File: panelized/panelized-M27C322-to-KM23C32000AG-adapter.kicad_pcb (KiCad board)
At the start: 2 copper layers, 115.5 x 108 mm, 544 parts, among them J1 PinSocket_2x22_P1.27mm_Vertic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, U1 KM23C32000AG-adaptor

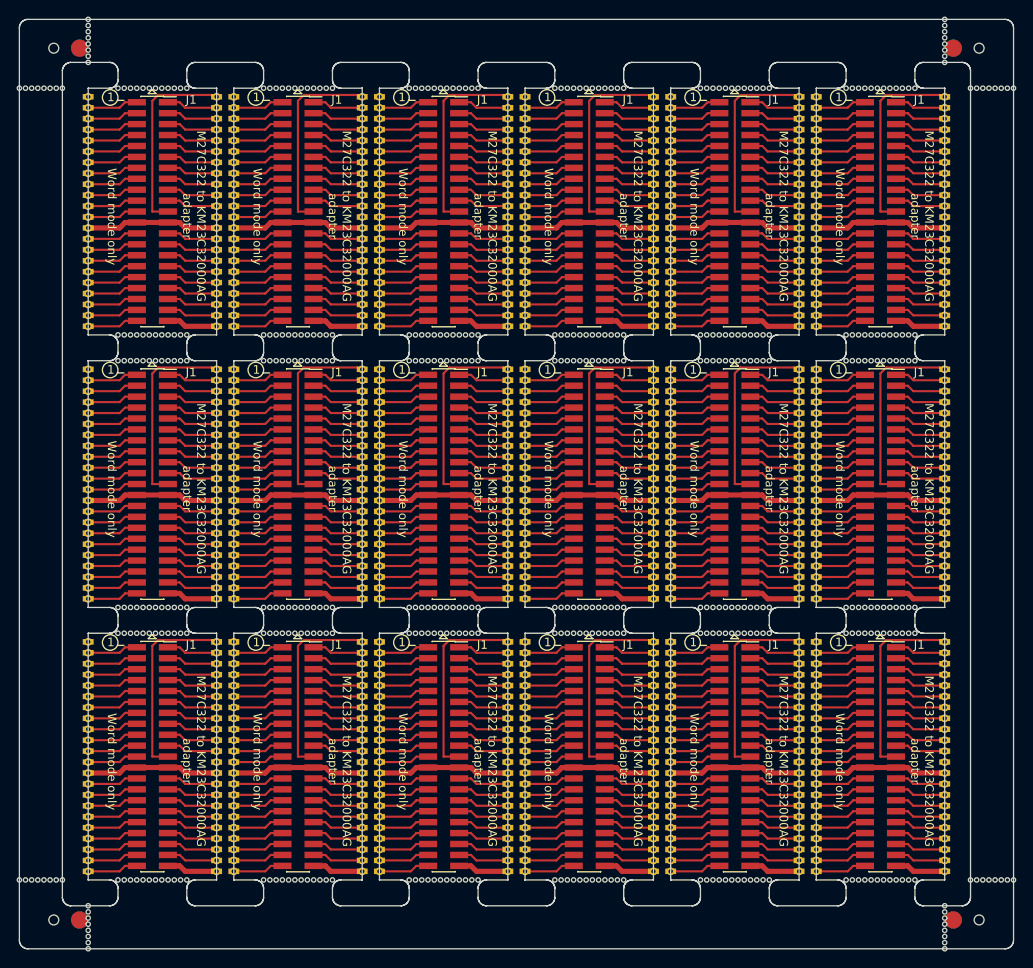
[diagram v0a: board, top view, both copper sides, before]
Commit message: WIP changes
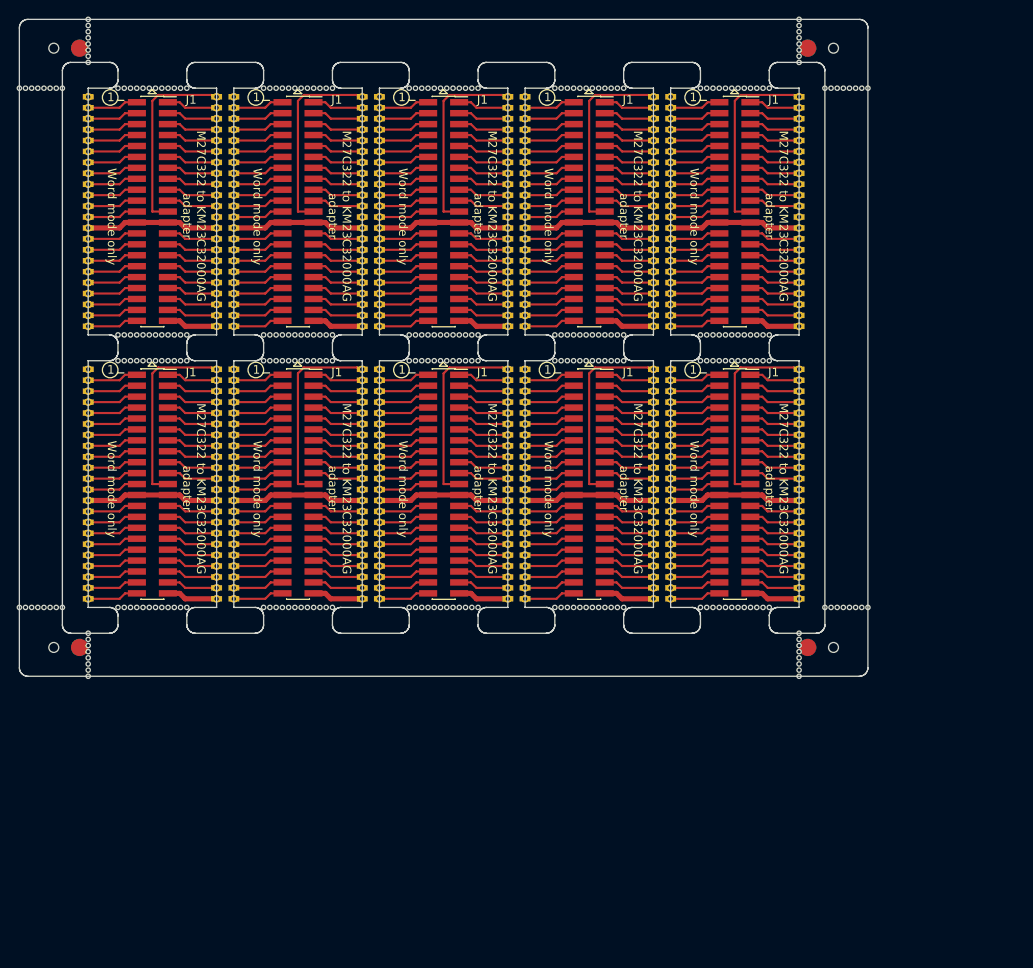
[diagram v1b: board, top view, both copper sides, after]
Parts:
- removed the J1 at (98.2, 100.7)
- removed the J1 at (115.1, 69.0)
- removed the J1 at (30.5, 100.7)
- removed the J1 at (64.3, 100.7)
- removed the J1 at (47.4, 100.7)
- removed the J1 at (81.2, 100.7)
- removed the J1 at (115.1, 37.3)
- removed the J1 at (115.1, 100.7)
- removed the REF** at (129.1, 23.0)
- removed the REF** at (85.2, 115.0)
- removed the REF** at (116.9, 115.0)
- removed the REF** at (122.5, 120.2)
- removed the REF** at (83.8, 115.0)
- removed the REF** at (28.6, 115.0)
- removed the REF** at (78.0, 115.0)
- removed the REF** at (100.7, 86.3)
- removed the REF** at (115.4, 51.7)
- removed the REF** at (47.0, 115.0)
- removed the REF** at (116.9, 23.0)
- removed the REF** at (63.2, 86.3)
- removed the REF** at (122.5, 18.6)
- removed the REF** at (100.0, 86.3)
- removed the REF** at (60.3, 86.3)
- removed the REF** at (68.3, 115.0)
- removed the REF** at (65.4, 86.3)
- removed the REF** at (111.1, 23.0)
- removed the REF** at (114.0, 51.7)
- removed the REF** at (64.7, 115.0)
- removed the REF** at (81.6, 86.3)
- removed the REF** at (94.2, 86.3)
- removed the REF** at (63.9, 86.3)
- removed the REF** at (114.7, 23.0)
- removed the REF** at (50.7, 86.3)
- removed the REF** at (128.4, 23.0)
- removed the REF** at (66.9, 115.0)
- removed the REF** at (112.5, 51.7)
- removed the REF** at (61.0, 86.3)
- removed the REF** at (118.3, 51.7)
- removed the REF** at (19.0, 119.7)
- removed the REF** at (22.0, 18.4) (x2)
- removed the REF** at (123.5, 18.4) (x2)
- removed the REF** at (33.7, 86.3)
- removed the REF** at (66.9, 86.3)
- removed the REF** at (111.8, 115.0)
- removed the REF** at (111.8, 51.7)
- removed the REF** at (112.5, 86.3)
- removed the REF** at (113.3, 23.0)
- removed the REF** at (49.2, 115.0)
- removed the REF** at (68.3, 86.3)
- removed the REF** at (116.9, 86.3)
- removed the REF** at (47.7, 115.0)
- removed the REF** at (115.4, 23.0)
- removed the REF** at (114.0, 115.0)
- removed the REF** at (61.0, 115.0)
- removed the REF** at (102.2, 115.0)
- removed the REF** at (77.2, 115.0)
- removed the REF** at (95.6, 115.0)
- removed the REF** at (98.5, 115.0)
- removed the REF** at (83.0, 115.0)
- removed the REF** at (30.8, 115.0)
- removed the REF** at (48.5, 86.3)
- removed the REF** at (119.1, 51.7)
- removed the REF** at (126.2, 115.0)
- removed the REF** at (119.1, 86.3)
- removed the REF** at (23.0, 123.0)
- removed the REF** at (126.5, 18.4)
- removed the REF** at (45.6, 86.3)
- removed the REF** at (32.3, 115.0)
- removed the REF** at (111.8, 23.0)
- removed the REF** at (51.4, 86.3)
- removed the REF** at (114.0, 54.7)
- removed the REF** at (23.0, 120.2)
- removed the REF** at (114.0, 86.3)
- removed the REF** at (79.4, 86.3)
- removed the REF** at (111.1, 115.0)
- removed the REF** at (117.6, 86.3)
- removed the REF** at (79.4, 115.0)
- removed the REF** at (117.6, 51.7)
- removed the REF** at (63.2, 115.0)
- removed the REF** at (113.3, 51.7)
- removed the REF** at (48.5, 115.0)
- removed the REF** at (94.2, 115.0)
- removed the REF** at (15.0, 115.0)
- removed the REF** at (27.2, 115.0)
- removed the REF** at (116.9, 54.7)
- removed the REF** at (118.3, 86.3)
- removed the REF** at (116.2, 54.7)
- removed the REF** at (122.5, 118.0)
- removed the REF** at (81.6, 115.0)
- removed the REF** at (22.0, 119.7) (x2)
- removed the REF** at (18.6, 115.0)
- removed the REF** at (112.5, 23.0)
- removed the REF** at (130.5, 23.0)
- removed the REF** at (34.5, 115.0)
- removed the REF** at (85.2, 86.3)
- removed the REF** at (127.0, 23.0)
- removed the REF** at (117.6, 83.3)
- removed the REF** at (49.9, 115.0)
- removed the REF** at (80.9, 86.3)
- removed the REF** at (27.2, 86.3)
- removed the REF** at (82.3, 86.3)
- removed the REF** at (61.8, 86.3)
- removed the REF** at (63.9, 115.0)
- removed the REF** at (100.7, 115.0)
- removed the REF** at (122.5, 120.9)
- removed the REF** at (128.4, 115.0)
- removed the REF** at (78.7, 115.0)
- removed the REF** at (16.4, 115.0)
- removed the REF** at (32.3, 86.3)
- removed the REF** at (64.7, 86.3)
- removed the REF** at (122.5, 17.9)
- removed the REF** at (114.7, 86.3)
- removed the REF** at (31.6, 86.3)
- removed the REF** at (127.7, 23.0)
- removed the REF** at (51.4, 115.0)
- removed the REF** at (119.1, 115.0)
- removed the REF** at (111.1, 54.7)
- removed the REF** at (112.5, 54.7)
- removed the REF** at (119.1, 83.3)
- removed the REF** at (47.0, 86.3)
- removed the REF** at (111.1, 86.3)
- removed the REF** at (46.3, 115.0)
- removed the REF** at (96.3, 115.0)
- removed the REF** at (23.0, 122.3)
- removed the REF** at (78.7, 86.3)
- removed the REF** at (114.7, 51.7)
- removed the REF** at (84.5, 86.3)
- removed the REF** at (114.7, 115.0)
- removed the REF** at (122.5, 15.0)
- removed the REF** at (80.1, 86.3)
- removed the REF** at (116.9, 83.3)
- removed the REF** at (99.2, 115.0)
- removed the REF** at (113.3, 115.0)
- removed the REF** at (122.5, 121.6)
- removed the REF** at (80.1, 115.0)
- removed the REF** at (65.4, 115.0)
- removed the REF** at (78.0, 86.3)
- removed the REF** at (95.6, 86.3)
- removed the REF** at (98.5, 86.3)
- removed the REF** at (119.1, 23.0)
- removed the REF** at (118.3, 23.0)
- removed the REF** at (27.9, 115.0)
- removed the REF** at (118.3, 83.3)
- removed the REF** at (29.4, 86.3)
- removed the REF** at (97.1, 115.0)
- removed the REF** at (17.1, 115.0)
- removed the REF** at (115.4, 86.3)
- removed the REF** at (43.4, 115.0)
- removed the REF** at (111.8, 54.7)
- removed the REF** at (34.5, 86.3)
- removed the REF** at (114.0, 23.0)
- removed the REF** at (116.2, 115.0)
- removed the REF** at (119.1, 54.7)
- removed the REF** at (125.5, 23.0)
- removed the REF** at (111.1, 83.3)
- removed the REF** at (116.2, 51.7)
- removed the REF** at (129.8, 115.0)
- removed the REF** at (99.2, 86.3)
- removed the REF** at (23.0, 118.0)
- removed the REF** at (116.2, 83.3)
- removed the REF** at (46.3, 86.3)
- removed the REF** at (66.1, 86.3)
- removed the REF** at (23.0, 120.9)
- removed the REF** at (96.3, 86.3)
- removed the REF** at (84.5, 115.0)
- removed the REF** at (82.3, 115.0)
- removed the REF** at (115.4, 83.3)
- removed the REF** at (112.5, 115.0)
- removed the REF** at (122.5, 20.0)
- removed the REF** at (23.0, 119.4)
- removed the REF** at (122.5, 119.4)
- removed the REF** at (97.8, 115.0)
- removed the REF** at (94.9, 86.3)
- removed the REF** at (47.7, 86.3)
- removed the REF** at (129.8, 23.0)
- removed the REF** at (67.6, 115.0)
- removed the REF** at (122.5, 16.4)
- removed the REF** at (111.8, 86.3)
- removed the REF** at (17.9, 115.0)
- removed the REF** at (62.5, 115.0)
- removed the REF** at (126.5, 119.7)
- removed the REF** at (30.1, 115.0)
- removed the REF** at (113.3, 54.7)
- removed the REF** at (127.7, 115.0)
- removed the REF** at (77.2, 86.3)
- removed the REF** at (44.8, 86.3)
- removed the REF** at (114.7, 83.3)
- removed the REF** at (114.7, 54.7)
- removed the REF** at (122.5, 15.7)
- removed the REF** at (115.4, 54.7)
- removed the REF** at (15.7, 115.0)
- removed the REF** at (23.0, 121.6)
- removed the REF** at (116.2, 23.0)
- removed the REF** at (129.1, 115.0)
- removed the REF** at (33.7, 115.0)
- removed the REF** at (20.0, 115.0)
- removed the REF** at (125.5, 115.0)
- removed the REF** at (50.7, 115.0)
- removed the REF** at (112.5, 83.3)
- removed the REF** at (94.9, 115.0)
- removed the REF** at (115.4, 115.0)
- removed the REF** at (97.8, 86.3)
- removed the REF** at (100.0, 115.0)
- removed the REF** at (66.1, 115.0)
- removed the REF** at (33.0, 86.3)
- removed the REF** at (83.8, 86.3)
- removed the REF** at (43.4, 86.3)
- removed the REF** at (26.5, 86.3)
- removed the REF** at (26.5, 115.0)
- removed the REF** at (97.1, 86.3)
- removed the REF** at (33.0, 115.0)
- removed the REF** at (101.4, 86.3)
- removed the REF** at (28.6, 86.3)
- removed the REF** at (29.4, 115.0)
- removed the REF** at (122.5, 123.0)
- removed the REF** at (114.0, 83.3)
- removed the REF** at (122.5, 122.3)
- removed the REF** at (31.6, 115.0)
- removed the REF** at (116.9, 51.7)
- removed the REF** at (127.0, 115.0)
- removed the REF** at (117.6, 115.0)
- removed the REF** at (102.2, 86.3)
- removed the REF** at (113.3, 86.3)
- removed the REF** at (62.5, 86.3)
- removed the REF** at (118.3, 115.0)
- removed the REF** at (122.5, 17.1)
- removed the REF** at (60.3, 115.0)
- removed the REF** at (27.9, 86.3)
- removed the REF** at (118.3, 54.7)
- removed the REF** at (116.2, 86.3)
- removed the REF** at (61.8, 115.0)
- removed the REF** at (123.5, 119.7) (x2)
- removed the REF** at (49.9, 86.3)
- removed the REF** at (101.4, 115.0)
- removed the REF** at (80.9, 115.0)
- removed the REF** at (44.1, 115.0)
- removed the REF** at (23.0, 118.7)
- removed the REF** at (122.5, 19.3)
- removed the REF** at (44.8, 115.0)
- removed the REF** at (49.2, 86.3)
- removed the REF** at (44.1, 86.3)
- removed the REF** at (113.3, 83.3)
- removed the REF** at (130.5, 115.0)
- removed the REF** at (126.2, 23.0)
- removed the REF** at (83.0, 86.3)
- removed the REF** at (111.8, 83.3)
- removed the REF** at (111.1, 51.7)
- removed the REF** at (117.6, 54.7)
- removed the REF** at (117.6, 23.0)
- removed the REF** at (19.3, 115.0)
- removed the REF** at (30.1, 86.3)
- removed the REF** at (45.6, 115.0)
- removed the REF** at (67.6, 86.3)
- removed the REF** at (122.5, 118.7)
- removed the REF** at (30.8, 86.3)
- removed the U1 at (115.1, 69.0)
- removed the U1 at (47.4, 100.7)
- removed the U1 at (115.1, 100.7)
- removed the U1 at (30.5, 100.7)
- removed the U1 at (98.2, 100.7)
- removed the U1 at (64.3, 100.7)
- removed the U1 at (81.2, 100.7)
- removed the U1 at (115.1, 37.3)
- added REF**: NPTH, NPTH, F.Cu at (108.6, 83.3)
- added REF**: NPTH, NPTH, F.Cu at (105.6, 87.1)
- added REF**: NPTH, NPTH, F.Cu at (105.6, 86.3)
- added REF**: NPTH, NPTH, F.Cu at (23.0, 90.6)
- added REF**: NPTH, NPTH, F.Cu at (110.8, 23.0)
- added REF**: NPTH, NPTH, F.Cu at (109.3, 83.3)
- added REF**: NPTH, NPTH, F.Cu at (112.9, 23.0)
- added REF**: NPTH, NPTH, F.Cu at (105.6, 89.9)
- added REF**: NPTH, NPTH, F.Cu at (23.0, 87.1)
- added REF**: NPTH, NPTH, F.Cu at (110.0, 23.0)
- added REF**: NPTH, NPTH, F.Cu at (16.4, 83.3)
- added REF**: Fiducial, Fiducial, F.Cu at (22.0, 88.0)
- added REF**: NPTH, NPTH, F.Cu at (109.6, 18.4)
- added REF**: NPTH, NPTH, F.Cu at (23.0, 87.8)
- added REF**: NPTH, NPTH, F.Cu at (105.6, 16.4)
- added REF**: NPTH, NPTH, F.Cu at (111.5, 83.3)
- added REF**: NPTH, NPTH, F.Cu at (105.6, 17.1)
- added REF**: NPTH, NPTH, F.Cu at (105.6, 20.0)
- added REF**: Fiducial, Fiducial, F.Cu at (22.0, 18.4)
- added REF**: NPTH, NPTH, F.Cu at (108.6, 23.0)
- added REF**: Fiducial, Fiducial, F.Cu at (106.6, 18.4)
- added REF**: NPTH, NPTH, F.Cu at (112.2, 23.0)
- added REF**: NPTH, NPTH, F.Cu at (110.8, 83.3)
- added REF**: NPTH, NPTH, F.Cu at (18.6, 83.3)
- added REF**: NPTH, NPTH, F.Cu at (105.6, 17.9)
- added REF**: NPTH, NPTH, F.Cu at (105.6, 90.6)
- added REF**: NPTH, NPTH, F.Cu at (17.9, 83.3)
- added REF**: NPTH, NPTH, F.Cu at (110.0, 83.3)
- added REF**: NPTH, NPTH, F.Cu at (109.3, 23.0)
- added REF**: NPTH, NPTH, F.Cu at (109.6, 88.0)
- added REF**: NPTH, NPTH, F.Cu at (20.0, 83.3)
- added REF**: NPTH, NPTH, F.Cu at (105.6, 15.0)
- added REF**: NPTH, NPTH, F.Cu at (19.3, 83.3)
- added REF**: NPTH, NPTH, F.Cu at (113.6, 23.0)
- added REF**: NPTH, NPTH, F.Cu at (17.1, 83.3)
- added REF**: NPTH, NPTH, F.Cu at (23.0, 89.9)
- added REF**: NPTH, NPTH, F.Cu at (23.0, 86.3)
- added REF**: NPTH, NPTH, F.Cu at (105.6, 88.5)
- added REF**: NPTH, NPTH, F.Cu at (23.0, 91.3)
- added REF**: NPTH, NPTH, F.Cu at (105.6, 19.3)
- added REF**: NPTH, NPTH, F.Cu at (105.6, 18.6)
- added REF**: Fiducial, Fiducial, B.Cu at (22.0, 18.4)
- added REF**: Fiducial, Fiducial, B.Cu at (106.6, 88.0)
- added REF**: Fiducial, Fiducial, B.Cu at (106.6, 18.4)
- added REF**: Fiducial, Fiducial, B.Cu at (22.0, 88.0)
- added REF**: NPTH, NPTH, F.Cu at (23.0, 89.2)
- added REF**: NPTH, NPTH, F.Cu at (113.6, 83.3)
- added REF**: NPTH, NPTH, F.Cu at (111.5, 23.0)
- added REF**: NPTH, NPTH, F.Cu at (15.0, 83.3)
- added REF**: NPTH, NPTH, F.Cu at (105.6, 15.7)
- added REF**: NPTH, NPTH, F.Cu at (19.0, 88.0)
- added REF**: NPTH, NPTH, F.Cu at (112.9, 83.3)
- added REF**: NPTH, NPTH, F.Cu at (112.2, 83.3)
- added REF**: NPTH, NPTH, F.Cu at (23.0, 88.5)
- added REF**: NPTH, NPTH, F.Cu at (105.6, 87.8)
- added REF**: NPTH, NPTH, F.Cu at (15.7, 83.3)
- added REF**: NPTH, NPTH, F.Cu at (105.6, 89.2)
- added REF**: Fiducial, Fiducial, F.Cu at (106.6, 88.0)
- added REF**: NPTH, NPTH, F.Cu at (105.6, 91.3)
- J1 (x10): value PinSocket_2x22_P1.27mm_Vertical -> PinSocket_2x21_P1.27mm_Vertical
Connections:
- J1 pad 1: Board_6-/A18 -> Board_5-/A18
- J1 pad 10: Board_6-/A0 -> Board_5-/A0
- J1 pad 11: Board_6-/~{CE} -> Board_5-/~{CE}
- J1 pad 12: Board_6-/VSS -> Board_5-/VSS
- J1 pad 13: Board_6-/~{OE} -> Board_5-/~{OE}
- J1 pad 14: Board_6-/D0 -> Board_5-/D0
- J1 pad 15: Board_6-/D8 -> Board_5-/D8
- J1 pad 16: Board_6-/D1 -> Board_5-/D1
- J1 pad 17: Board_6-/D9 -> Board_5-/D9
- J1 pad 18: Board_6-/D2 -> Board_5-/D2
- J1 pad 19: Board_6-/D10 -> Board_5-/D10
- J1 pad 2: Board_6-/A17 -> Board_5-/A17
- J1 pad 20: Board_6-/D3 -> Board_5-/D3
- J1 pad 21: Board_6-/D11 -> Board_5-/D11
- J1 pad 22: Board_6-/VCC -> Board_5-/VCC
- J1 pad 23: Board_6-/D4 -> Board_5-/D4
- J1 pad 24: Board_6-/D12 -> Board_5-/D12
- J1 pad 25: Board_6-/D5 -> Board_5-/D5
- J1 pad 26: Board_6-/D13 -> Board_5-/D13
- J1 pad 27: Board_6-/D6 -> Board_5-/D6
- J1 pad 28: Board_6-/D14 -> Board_5-/D14
- J1 pad 29: Board_6-/D7 -> Board_5-/D7
- J1 pad 3: Board_6-/A7 -> Board_5-/A7
- J1 pad 30: Board_6-/D15 -> Board_5-/D15
- J1 pad 31: Board_6-/VSS -> Board_5-/VSS
- J1 pad 32: Board_6-/A20 -> Board_5-/A20
- J1 pad 33: Board_6-/A16 -> Board_5-/A16
- J1 pad 34: Board_6-/A15 -> Board_5-/A15
- J1 pad 35: Board_6-/A14 -> Board_5-/A14
- J1 pad 36: Board_6-/A13 -> Board_5-/A13
- J1 pad 37: Board_6-/A12 -> Board_5-/A12
- J1 pad 38: Board_6-/A11 -> Board_5-/A11
- J1 pad 39: Board_6-/A10 -> Board_5-/A10
- J1 pad 4: Board_6-/A6 -> Board_5-/A6
- J1 pad 40: Board_6-/A9 -> Board_5-/A9
- J1 pad 41: Board_6-/A8 -> Board_5-/A8
- J1 pad 42: Board_6-/A19 -> Board_5-/A19
- J1 pad 5: Board_6-/A5 -> Board_5-/A5
- J1 pad 6: Board_6-/A4 -> Board_5-/A4
- J1 pad 7: Board_6-/A3 -> Board_5-/A3
- J1 pad 8: Board_6-/A2 -> Board_5-/A2
- J1 pad 9: Board_6-/A1 -> Board_5-/A1
- J1 pad 1: Board_9-/A18 -> Board_8-/A18
- J1 pad 10: Board_9-/A0 -> Board_8-/A0
- J1 pad 11: Board_9-/~{CE} -> Board_8-/~{CE}
- J1 pad 12: Board_9-/VSS -> Board_8-/VSS
- J1 pad 13: Board_9-/~{OE} -> Board_8-/~{OE}
- J1 pad 14: Board_9-/D0 -> Board_8-/D0
- J1 pad 15: Board_9-/D8 -> Board_8-/D8
- J1 pad 16: Board_9-/D1 -> Board_8-/D1
- J1 pad 17: Board_9-/D9 -> Board_8-/D9
- J1 pad 18: Board_9-/D2 -> Board_8-/D2
- J1 pad 19: Board_9-/D10 -> Board_8-/D10
- J1 pad 2: Board_9-/A17 -> Board_8-/A17
- J1 pad 20: Board_9-/D3 -> Board_8-/D3
- J1 pad 21: Board_9-/D11 -> Board_8-/D11
- J1 pad 22: Board_9-/VCC -> Board_8-/VCC
- J1 pad 23: Board_9-/D4 -> Board_8-/D4
- J1 pad 24: Board_9-/D12 -> Board_8-/D12
- J1 pad 25: Board_9-/D5 -> Board_8-/D5
- J1 pad 26: Board_9-/D13 -> Board_8-/D13
- J1 pad 27: Board_9-/D6 -> Board_8-/D6
- J1 pad 28: Board_9-/D14 -> Board_8-/D14
- J1 pad 29: Board_9-/D7 -> Board_8-/D7
- J1 pad 3: Board_9-/A7 -> Board_8-/A7
- J1 pad 30: Board_9-/D15 -> Board_8-/D15
- J1 pad 31: Board_9-/VSS -> Board_8-/VSS
- J1 pad 32: Board_9-/A20 -> Board_8-/A20
- J1 pad 33: Board_9-/A16 -> Board_8-/A16
- J1 pad 34: Board_9-/A15 -> Board_8-/A15
- J1 pad 35: Board_9-/A14 -> Board_8-/A14
- J1 pad 36: Board_9-/A13 -> Board_8-/A13
- J1 pad 37: Board_9-/A12 -> Board_8-/A12
- J1 pad 38: Board_9-/A11 -> Board_8-/A11
- J1 pad 39: Board_9-/A10 -> Board_8-/A10
- J1 pad 4: Board_9-/A6 -> Board_8-/A6
- J1 pad 40: Board_9-/A9 -> Board_8-/A9
- J1 pad 41: Board_9-/A8 -> Board_8-/A8
- J1 pad 42: Board_9-/A19 -> Board_8-/A19
- J1 pad 5: Board_9-/A5 -> Board_8-/A5
- J1 pad 6: Board_9-/A4 -> Board_8-/A4
- J1 pad 7: Board_9-/A3 -> Board_8-/A3
- J1 pad 8: Board_9-/A2 -> Board_8-/A2
- J1 pad 9: Board_9-/A1 -> Board_8-/A1
- J1 pad 1: Board_7-/A18 -> Board_6-/A18
- J1 pad 10: Board_7-/A0 -> Board_6-/A0
- J1 pad 11: Board_7-/~{CE} -> Board_6-/~{CE}
- J1 pad 12: Board_7-/VSS -> Board_6-/VSS
- J1 pad 13: Board_7-/~{OE} -> Board_6-/~{OE}
- J1 pad 14: Board_7-/D0 -> Board_6-/D0
- J1 pad 15: Board_7-/D8 -> Board_6-/D8
- J1 pad 16: Board_7-/D1 -> Board_6-/D1
- J1 pad 17: Board_7-/D9 -> Board_6-/D9
- J1 pad 18: Board_7-/D2 -> Board_6-/D2
- J1 pad 19: Board_7-/D10 -> Board_6-/D10
- J1 pad 2: Board_7-/A17 -> Board_6-/A17
- J1 pad 20: Board_7-/D3 -> Board_6-/D3
- J1 pad 21: Board_7-/D11 -> Board_6-/D11
- J1 pad 22: Board_7-/VCC -> Board_6-/VCC
- J1 pad 23: Board_7-/D4 -> Board_6-/D4
- J1 pad 24: Board_7-/D12 -> Board_6-/D12
- J1 pad 25: Board_7-/D5 -> Board_6-/D5
- J1 pad 26: Board_7-/D13 -> Board_6-/D13
- J1 pad 27: Board_7-/D6 -> Board_6-/D6
- J1 pad 28: Board_7-/D14 -> Board_6-/D14
- J1 pad 29: Board_7-/D7 -> Board_6-/D7
- J1 pad 3: Board_7-/A7 -> Board_6-/A7
- J1 pad 30: Board_7-/D15 -> Board_6-/D15
- J1 pad 31: Board_7-/VSS -> Board_6-/VSS
- J1 pad 32: Board_7-/A20 -> Board_6-/A20
- J1 pad 33: Board_7-/A16 -> Board_6-/A16
- J1 pad 34: Board_7-/A15 -> Board_6-/A15
- J1 pad 35: Board_7-/A14 -> Board_6-/A14
- J1 pad 36: Board_7-/A13 -> Board_6-/A13
- J1 pad 37: Board_7-/A12 -> Board_6-/A12
- J1 pad 38: Board_7-/A11 -> Board_6-/A11
- J1 pad 39: Board_7-/A10 -> Board_6-/A10
- J1 pad 4: Board_7-/A6 -> Board_6-/A6
- J1 pad 40: Board_7-/A9 -> Board_6-/A9
- J1 pad 41: Board_7-/A8 -> Board_6-/A8
- J1 pad 42: Board_7-/A19 -> Board_6-/A19
- J1 pad 5: Board_7-/A5 -> Board_6-/A5
- J1 pad 6: Board_7-/A4 -> Board_6-/A4
- J1 pad 7: Board_7-/A3 -> Board_6-/A3
- J1 pad 8: Board_7-/A2 -> Board_6-/A2
- J1 pad 9: Board_7-/A1 -> Board_6-/A1
- J1 pad 1: Board_10-/A18 -> Board_9-/A18
- J1 pad 10: Board_10-/A0 -> Board_9-/A0
- J1 pad 11: Board_10-/~{CE} -> Board_9-/~{CE}
- J1 pad 12: Board_10-/VSS -> Board_9-/VSS
- J1 pad 13: Board_10-/~{OE} -> Board_9-/~{OE}
- J1 pad 14: Board_10-/D0 -> Board_9-/D0
- J1 pad 15: Board_10-/D8 -> Board_9-/D8
- J1 pad 16: Board_10-/D1 -> Board_9-/D1
- J1 pad 17: Board_10-/D9 -> Board_9-/D9
- J1 pad 18: Board_10-/D2 -> Board_9-/D2
- J1 pad 19: Board_10-/D10 -> Board_9-/D10
- J1 pad 2: Board_10-/A17 -> Board_9-/A17
- J1 pad 20: Board_10-/D3 -> Board_9-/D3
- J1 pad 21: Board_10-/D11 -> Board_9-/D11
- J1 pad 22: Board_10-/VCC -> Board_9-/VCC
- J1 pad 23: Board_10-/D4 -> Board_9-/D4
- J1 pad 24: Board_10-/D12 -> Board_9-/D12
- J1 pad 25: Board_10-/D5 -> Board_9-/D5
- J1 pad 26: Board_10-/D13 -> Board_9-/D13
- J1 pad 27: Board_10-/D6 -> Board_9-/D6
- J1 pad 28: Board_10-/D14 -> Board_9-/D14
- J1 pad 29: Board_10-/D7 -> Board_9-/D7
- J1 pad 3: Board_10-/A7 -> Board_9-/A7
- J1 pad 30: Board_10-/D15 -> Board_9-/D15
- J1 pad 31: Board_10-/VSS -> Board_9-/VSS
- J1 pad 32: Board_10-/A20 -> Board_9-/A20
- J1 pad 33: Board_10-/A16 -> Board_9-/A16
- J1 pad 34: Board_10-/A15 -> Board_9-/A15
- J1 pad 35: Board_10-/A14 -> Board_9-/A14
- J1 pad 36: Board_10-/A13 -> Board_9-/A13
- J1 pad 37: Board_10-/A12 -> Board_9-/A12
- J1 pad 38: Board_10-/A11 -> Board_9-/A11
- J1 pad 39: Board_10-/A10 -> Board_9-/A10
- J1 pad 4: Board_10-/A6 -> Board_9-/A6
- J1 pad 40: Board_10-/A9 -> Board_9-/A9
- J1 pad 41: Board_10-/A8 -> Board_9-/A8
- J1 pad 42: Board_10-/A19 -> Board_9-/A19
- J1 pad 5: Board_10-/A5 -> Board_9-/A5
- J1 pad 6: Board_10-/A4 -> Board_9-/A4
- J1 pad 7: Board_10-/A3 -> Board_9-/A3
- J1 pad 8: Board_10-/A2 -> Board_9-/A2
- J1 pad 9: Board_10-/A1 -> Board_9-/A1
- J1 pad 1: Board_8-/A18 -> Board_7-/A18
- J1 pad 10: Board_8-/A0 -> Board_7-/A0
- J1 pad 11: Board_8-/~{CE} -> Board_7-/~{CE}
- J1 pad 12: Board_8-/VSS -> Board_7-/VSS
- J1 pad 13: Board_8-/~{OE} -> Board_7-/~{OE}
- J1 pad 14: Board_8-/D0 -> Board_7-/D0
- J1 pad 15: Board_8-/D8 -> Board_7-/D8
- J1 pad 16: Board_8-/D1 -> Board_7-/D1
- J1 pad 17: Board_8-/D9 -> Board_7-/D9
- J1 pad 18: Board_8-/D2 -> Board_7-/D2
- J1 pad 19: Board_8-/D10 -> Board_7-/D10
- J1 pad 2: Board_8-/A17 -> Board_7-/A17
- J1 pad 20: Board_8-/D3 -> Board_7-/D3
- J1 pad 21: Board_8-/D11 -> Board_7-/D11
- J1 pad 22: Board_8-/VCC -> Board_7-/VCC
- J1 pad 23: Board_8-/D4 -> Board_7-/D4
- J1 pad 24: Board_8-/D12 -> Board_7-/D12
- J1 pad 25: Board_8-/D5 -> Board_7-/D5
- J1 pad 26: Board_8-/D13 -> Board_7-/D13
- J1 pad 27: Board_8-/D6 -> Board_7-/D6
- J1 pad 28: Board_8-/D14 -> Board_7-/D14
- J1 pad 29: Board_8-/D7 -> Board_7-/D7
- J1 pad 3: Board_8-/A7 -> Board_7-/A7
- J1 pad 30: Board_8-/D15 -> Board_7-/D15
- J1 pad 31: Board_8-/VSS -> Board_7-/VSS
- J1 pad 32: Board_8-/A20 -> Board_7-/A20
- J1 pad 33: Board_8-/A16 -> Board_7-/A16
- J1 pad 34: Board_8-/A15 -> Board_7-/A15
- J1 pad 35: Board_8-/A14 -> Board_7-/A14
- J1 pad 36: Board_8-/A13 -> Board_7-/A13
- J1 pad 37: Board_8-/A12 -> Board_7-/A12
- J1 pad 38: Board_8-/A11 -> Board_7-/A11
- J1 pad 39: Board_8-/A10 -> Board_7-/A10
- J1 pad 4: Board_8-/A6 -> Board_7-/A6
- J1 pad 40: Board_8-/A9 -> Board_7-/A9
- J1 pad 41: Board_8-/A8 -> Board_7-/A8
- J1 pad 42: Board_8-/A19 -> Board_7-/A19
- J1 pad 5: Board_8-/A5 -> Board_7-/A5
- J1 pad 6: Board_8-/A4 -> Board_7-/A4
- J1 pad 7: Board_8-/A3 -> Board_7-/A3
- J1 pad 8: Board_8-/A2 -> Board_7-/A2
- J1 pad 9: Board_8-/A1 -> Board_7-/A1
- U1 pad 1: Board_9-unconnected-(U1-Pad1) -> Board_8-unconnected-(U1-Pad1)
- U1 pad 10: Board_9-/A1 -> Board_8-/A1
- U1 pad 11: Board_9-/A0 -> Board_8-/A0
- U1 pad 12: Board_9-/~{CE} -> Board_8-/~{CE}
- U1 pad 13: Board_9-/VSS -> Board_8-/VSS
- U1 pad 14: Board_9-/~{OE} -> Board_8-/~{OE}
- U1 pad 15: Board_9-/D0 -> Board_8-/D0
- U1 pad 16: Board_9-/D8 -> Board_8-/D8
- U1 pad 17: Board_9-/D1 -> Board_8-/D1
- U1 pad 18: Board_9-/D9 -> Board_8-/D9
- U1 pad 19: Board_9-/D2 -> Board_8-/D2
- U1 pad 2: Board_9-/A18 -> Board_8-/A18
- U1 pad 20: Board_9-/D10 -> Board_8-/D10
- U1 pad 21: Board_9-/D3 -> Board_8-/D3
- U1 pad 22: Board_9-/D11 -> Board_8-/D11
- U1 pad 23: Board_9-/VCC -> Board_8-/VCC
- U1 pad 24: Board_9-/D4 -> Board_8-/D4
- U1 pad 25: Board_9-/D12 -> Board_8-/D12
- U1 pad 26: Board_9-/D5 -> Board_8-/D5
- U1 pad 27: Board_9-/D13 -> Board_8-/D13
- U1 pad 28: Board_9-/D6 -> Board_8-/D6
- U1 pad 29: Board_9-/D14 -> Board_8-/D14
- U1 pad 3: Board_9-/A17 -> Board_8-/A17
- U1 pad 30: Board_9-/D7 -> Board_8-/D7
- U1 pad 31: Board_9-/D15 -> Board_8-/D15
- U1 pad 32: Board_9-/VSS -> Board_8-/VSS
- U1 pad 33: Board_9-unconnected-(U1-Pad33) -> Board_8-unconnected-(U1-Pad33)
- U1 pad 34: Board_9-/A16 -> Board_8-/A16
- U1 pad 35: Board_9-/A15 -> Board_8-/A15
- U1 pad 36: Board_9-/A14 -> Board_8-/A14
- U1 pad 37: Board_9-/A13 -> Board_8-/A13
- U1 pad 38: Board_9-/A12 -> Board_8-/A12
- U1 pad 39: Board_9-/A11 -> Board_8-/A11
- U1 pad 4: Board_9-/A7 -> Board_8-/A7
- U1 pad 40: Board_9-/A10 -> Board_8-/A10
- U1 pad 41: Board_9-/A9 -> Board_8-/A9
- U1 pad 42: Board_9-/A8 -> Board_8-/A8
- U1 pad 43: Board_9-/A19 -> Board_8-/A19
- U1 pad 44: Board_9-/A20 -> Board_8-/A20
- U1 pad 5: Board_9-/A6 -> Board_8-/A6
- U1 pad 6: Board_9-/A5 -> Board_8-/A5
- U1 pad 7: Board_9-/A4 -> Board_8-/A4
- U1 pad 8: Board_9-/A3 -> Board_8-/A3
- U1 pad 9: Board_9-/A2 -> Board_8-/A2
- U1 pad 1: Board_10-unconnected-(U1-Pad1) -> Board_9-unconnected-(U1-Pad1)
- U1 pad 10: Board_10-/A1 -> Board_9-/A1
- U1 pad 11: Board_10-/A0 -> Board_9-/A0
- U1 pad 12: Board_10-/~{CE} -> Board_9-/~{CE}
- U1 pad 13: Board_10-/VSS -> Board_9-/VSS
- U1 pad 14: Board_10-/~{OE} -> Board_9-/~{OE}
- U1 pad 15: Board_10-/D0 -> Board_9-/D0
- U1 pad 16: Board_10-/D8 -> Board_9-/D8
- U1 pad 17: Board_10-/D1 -> Board_9-/D1
- U1 pad 18: Board_10-/D9 -> Board_9-/D9
- U1 pad 19: Board_10-/D2 -> Board_9-/D2
- U1 pad 2: Board_10-/A18 -> Board_9-/A18
- U1 pad 20: Board_10-/D10 -> Board_9-/D10
- U1 pad 21: Board_10-/D3 -> Board_9-/D3
- U1 pad 22: Board_10-/D11 -> Board_9-/D11
- U1 pad 23: Board_10-/VCC -> Board_9-/VCC
- U1 pad 24: Board_10-/D4 -> Board_9-/D4
- U1 pad 25: Board_10-/D12 -> Board_9-/D12
- U1 pad 26: Board_10-/D5 -> Board_9-/D5
- U1 pad 27: Board_10-/D13 -> Board_9-/D13
- U1 pad 28: Board_10-/D6 -> Board_9-/D6
- U1 pad 29: Board_10-/D14 -> Board_9-/D14
- U1 pad 3: Board_10-/A17 -> Board_9-/A17
- U1 pad 30: Board_10-/D7 -> Board_9-/D7
- U1 pad 31: Board_10-/D15 -> Board_9-/D15
- U1 pad 32: Board_10-/VSS -> Board_9-/VSS
- U1 pad 33: Board_10-unconnected-(U1-Pad33) -> Board_9-unconnected-(U1-Pad33)
- U1 pad 34: Board_10-/A16 -> Board_9-/A16
- U1 pad 35: Board_10-/A15 -> Board_9-/A15
- U1 pad 36: Board_10-/A14 -> Board_9-/A14
- U1 pad 37: Board_10-/A13 -> Board_9-/A13
- U1 pad 38: Board_10-/A12 -> Board_9-/A12
- U1 pad 39: Board_10-/A11 -> Board_9-/A11
- U1 pad 4: Board_10-/A7 -> Board_9-/A7
- U1 pad 40: Board_10-/A10 -> Board_9-/A10
- U1 pad 41: Board_10-/A9 -> Board_9-/A9
- U1 pad 42: Board_10-/A8 -> Board_9-/A8
- U1 pad 43: Board_10-/A19 -> Board_9-/A19
- U1 pad 44: Board_10-/A20 -> Board_9-/A20
- U1 pad 5: Board_10-/A6 -> Board_9-/A6
- U1 pad 6: Board_10-/A5 -> Board_9-/A5
- U1 pad 7: Board_10-/A4 -> Board_9-/A4
- U1 pad 8: Board_10-/A3 -> Board_9-/A3
- U1 pad 9: Board_10-/A2 -> Board_9-/A2
- U1 pad 1: Board_6-unconnected-(U1-Pad1) -> Board_5-unconnected-(U1-Pad1)
- U1 pad 10: Board_6-/A1 -> Board_5-/A1
- U1 pad 11: Board_6-/A0 -> Board_5-/A0
- U1 pad 12: Board_6-/~{CE} -> Board_5-/~{CE}
- U1 pad 13: Board_6-/VSS -> Board_5-/VSS
- U1 pad 14: Board_6-/~{OE} -> Board_5-/~{OE}
- U1 pad 15: Board_6-/D0 -> Board_5-/D0
- U1 pad 16: Board_6-/D8 -> Board_5-/D8
- U1 pad 17: Board_6-/D1 -> Board_5-/D1
- U1 pad 18: Board_6-/D9 -> Board_5-/D9
- U1 pad 19: Board_6-/D2 -> Board_5-/D2
- U1 pad 2: Board_6-/A18 -> Board_5-/A18
- U1 pad 20: Board_6-/D10 -> Board_5-/D10
- U1 pad 21: Board_6-/D3 -> Board_5-/D3
- U1 pad 22: Board_6-/D11 -> Board_5-/D11
- U1 pad 23: Board_6-/VCC -> Board_5-/VCC
- U1 pad 24: Board_6-/D4 -> Board_5-/D4
- U1 pad 25: Board_6-/D12 -> Board_5-/D12
- U1 pad 26: Board_6-/D5 -> Board_5-/D5
- U1 pad 27: Board_6-/D13 -> Board_5-/D13
- U1 pad 28: Board_6-/D6 -> Board_5-/D6
- U1 pad 29: Board_6-/D14 -> Board_5-/D14
- U1 pad 3: Board_6-/A17 -> Board_5-/A17
- U1 pad 30: Board_6-/D7 -> Board_5-/D7
- U1 pad 31: Board_6-/D15 -> Board_5-/D15
- U1 pad 32: Board_6-/VSS -> Board_5-/VSS
- U1 pad 33: Board_6-unconnected-(U1-Pad33) -> Board_5-unconnected-(U1-Pad33)
- U1 pad 34: Board_6-/A16 -> Board_5-/A16
- U1 pad 35: Board_6-/A15 -> Board_5-/A15
- U1 pad 36: Board_6-/A14 -> Board_5-/A14
- U1 pad 37: Board_6-/A13 -> Board_5-/A13
- U1 pad 38: Board_6-/A12 -> Board_5-/A12
- U1 pad 39: Board_6-/A11 -> Board_5-/A11
- U1 pad 4: Board_6-/A7 -> Board_5-/A7
- U1 pad 40: Board_6-/A10 -> Board_5-/A10
- U1 pad 41: Board_6-/A9 -> Board_5-/A9
- U1 pad 42: Board_6-/A8 -> Board_5-/A8
- U1 pad 43: Board_6-/A19 -> Board_5-/A19
- U1 pad 44: Board_6-/A20 -> Board_5-/A20
- U1 pad 5: Board_6-/A6 -> Board_5-/A6
- U1 pad 6: Board_6-/A5 -> Board_5-/A5
- U1 pad 7: Board_6-/A4 -> Board_5-/A4
- U1 pad 8: Board_6-/A3 -> Board_5-/A3
- U1 pad 9: Board_6-/A2 -> Board_5-/A2
- U1 pad 1: Board_8-unconnected-(U1-Pad1) -> Board_7-unconnected-(U1-Pad1)
- U1 pad 10: Board_8-/A1 -> Board_7-/A1
- U1 pad 11: Board_8-/A0 -> Board_7-/A0
- U1 pad 12: Board_8-/~{CE} -> Board_7-/~{CE}
- U1 pad 13: Board_8-/VSS -> Board_7-/VSS
- U1 pad 14: Board_8-/~{OE} -> Board_7-/~{OE}
- U1 pad 15: Board_8-/D0 -> Board_7-/D0
- U1 pad 16: Board_8-/D8 -> Board_7-/D8
- U1 pad 17: Board_8-/D1 -> Board_7-/D1
- U1 pad 18: Board_8-/D9 -> Board_7-/D9
- U1 pad 19: Board_8-/D2 -> Board_7-/D2
- U1 pad 2: Board_8-/A18 -> Board_7-/A18
- U1 pad 20: Board_8-/D10 -> Board_7-/D10
- U1 pad 21: Board_8-/D3 -> Board_7-/D3
- U1 pad 22: Board_8-/D11 -> Board_7-/D11
- U1 pad 23: Board_8-/VCC -> Board_7-/VCC
- U1 pad 24: Board_8-/D4 -> Board_7-/D4
- U1 pad 25: Board_8-/D12 -> Board_7-/D12
- U1 pad 26: Board_8-/D5 -> Board_7-/D5
- U1 pad 27: Board_8-/D13 -> Board_7-/D13
- U1 pad 28: Board_8-/D6 -> Board_7-/D6
- U1 pad 29: Board_8-/D14 -> Board_7-/D14
- U1 pad 3: Board_8-/A17 -> Board_7-/A17
- U1 pad 30: Board_8-/D7 -> Board_7-/D7
- U1 pad 31: Board_8-/D15 -> Board_7-/D15
- U1 pad 32: Board_8-/VSS -> Board_7-/VSS
- U1 pad 33: Board_8-unconnected-(U1-Pad33) -> Board_7-unconnected-(U1-Pad33)
- U1 pad 34: Board_8-/A16 -> Board_7-/A16
- U1 pad 35: Board_8-/A15 -> Board_7-/A15
- U1 pad 36: Board_8-/A14 -> Board_7-/A14
- U1 pad 37: Board_8-/A13 -> Board_7-/A13
- U1 pad 38: Board_8-/A12 -> Board_7-/A12
- U1 pad 39: Board_8-/A11 -> Board_7-/A11
- U1 pad 4: Board_8-/A7 -> Board_7-/A7
- U1 pad 40: Board_8-/A10 -> Board_7-/A10
- U1 pad 41: Board_8-/A9 -> Board_7-/A9
- U1 pad 42: Board_8-/A8 -> Board_7-/A8
- U1 pad 43: Board_8-/A19 -> Board_7-/A19
- U1 pad 44: Board_8-/A20 -> Board_7-/A20
- U1 pad 5: Board_8-/A6 -> Board_7-/A6
- U1 pad 6: Board_8-/A5 -> Board_7-/A5
- U1 pad 7: Board_8-/A4 -> Board_7-/A4
- U1 pad 8: Board_8-/A3 -> Board_7-/A3
- U1 pad 9: Board_8-/A2 -> Board_7-/A2
- U1 pad 1: Board_7-unconnected-(U1-Pad1) -> Board_6-unconnected-(U1-Pad1)
- U1 pad 10: Board_7-/A1 -> Board_6-/A1
- U1 pad 11: Board_7-/A0 -> Board_6-/A0
- U1 pad 12: Board_7-/~{CE} -> Board_6-/~{CE}
- U1 pad 13: Board_7-/VSS -> Board_6-/VSS
- U1 pad 14: Board_7-/~{OE} -> Board_6-/~{OE}
- U1 pad 15: Board_7-/D0 -> Board_6-/D0
- U1 pad 16: Board_7-/D8 -> Board_6-/D8
- U1 pad 17: Board_7-/D1 -> Board_6-/D1
- U1 pad 18: Board_7-/D9 -> Board_6-/D9
- U1 pad 19: Board_7-/D2 -> Board_6-/D2
- U1 pad 2: Board_7-/A18 -> Board_6-/A18
- U1 pad 20: Board_7-/D10 -> Board_6-/D10
- U1 pad 21: Board_7-/D3 -> Board_6-/D3
- U1 pad 22: Board_7-/D11 -> Board_6-/D11
- U1 pad 23: Board_7-/VCC -> Board_6-/VCC
- U1 pad 24: Board_7-/D4 -> Board_6-/D4
- U1 pad 25: Board_7-/D12 -> Board_6-/D12
- U1 pad 26: Board_7-/D5 -> Board_6-/D5
- U1 pad 27: Board_7-/D13 -> Board_6-/D13
- U1 pad 28: Board_7-/D6 -> Board_6-/D6
- U1 pad 29: Board_7-/D14 -> Board_6-/D14
- U1 pad 3: Board_7-/A17 -> Board_6-/A17
- U1 pad 30: Board_7-/D7 -> Board_6-/D7
- U1 pad 31: Board_7-/D15 -> Board_6-/D15
- U1 pad 32: Board_7-/VSS -> Board_6-/VSS
- U1 pad 33: Board_7-unconnected-(U1-Pad33) -> Board_6-unconnected-(U1-Pad33)
- U1 pad 34: Board_7-/A16 -> Board_6-/A16
- U1 pad 35: Board_7-/A15 -> Board_6-/A15
- U1 pad 36: Board_7-/A14 -> Board_6-/A14
- U1 pad 37: Board_7-/A13 -> Board_6-/A13
- U1 pad 38: Board_7-/A12 -> Board_6-/A12
- U1 pad 39: Board_7-/A11 -> Board_6-/A11
- U1 pad 4: Board_7-/A7 -> Board_6-/A7
- U1 pad 40: Board_7-/A10 -> Board_6-/A10
- U1 pad 41: Board_7-/A9 -> Board_6-/A9
- U1 pad 42: Board_7-/A8 -> Board_6-/A8
- U1 pad 43: Board_7-/A19 -> Board_6-/A19
- U1 pad 44: Board_7-/A20 -> Board_6-/A20
- U1 pad 5: Board_7-/A6 -> Board_6-/A6
- U1 pad 6: Board_7-/A5 -> Board_6-/A5
- U1 pad 7: Board_7-/A4 -> Board_6-/A4
- U1 pad 8: Board_7-/A3 -> Board_6-/A3
- U1 pad 9: Board_7-/A2 -> Board_6-/A2
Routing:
- net Board_11-/A20: track 22.1 -> 0.00 mm
- net Board_17-/A20: track 22.1 -> 0.00 mm
- net Board_13-/A20: track 22.1 -> 0.00 mm
- net Board_12-/A20: track 22.1 -> 0.00 mm
- net Board_10-/A20: track 22.1 -> 0.00 mm
- net Board_16-/A20: track 22.1 -> 0.00 mm
- net Board_15-/A20: track 22.1 -> 0.00 mm
- net Board_14-/A20: track 22.1 -> 0.00 mm
- net Board_13-/VSS: track 14.2 -> 0.00 mm
- net Board_12-/VSS: track 14.2 -> 0.00 mm
- net Board_14-/VSS: track 14.2 -> 0.00 mm
- net Board_17-/VSS: track 14.2 -> 0.00 mm
- net Board_16-/VSS: track 14.2 -> 0.00 mm
- net Board_15-/VSS: track 14.2 -> 0.00 mm
- net Board_11-/VSS: track 14.2 -> 0.00 mm
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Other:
- board size 115.5 x 108 mm -> 98.6 x 76.3 mm
